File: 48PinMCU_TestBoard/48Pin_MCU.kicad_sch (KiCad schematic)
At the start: 33 parts, among them IC1 74LVC1G157GW,125, J4 SWD, J5 SWD, SW1 Reset, SW2 SW_SPDT, U1 STM32G431CBT6, Y1 Crystal

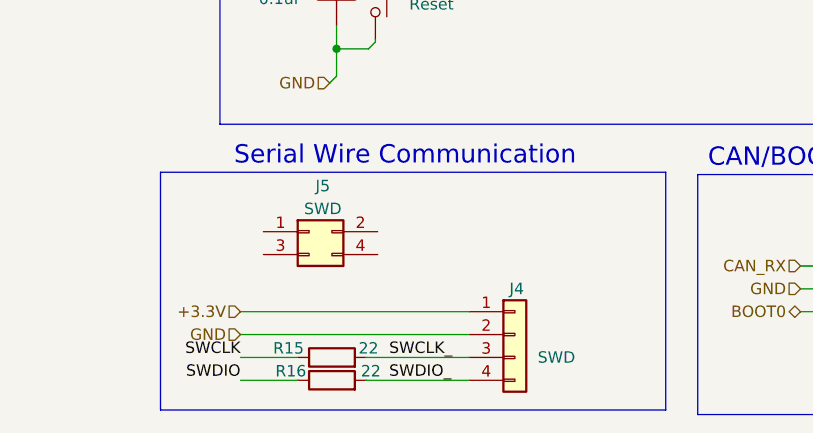
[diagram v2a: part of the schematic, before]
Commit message: made more changes!!
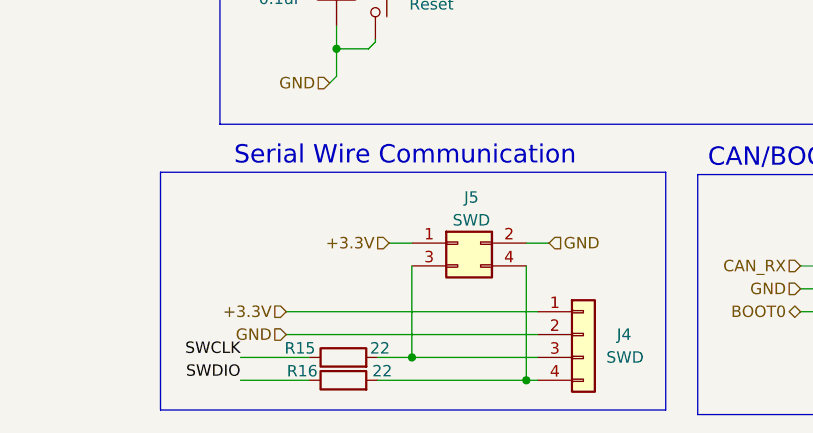
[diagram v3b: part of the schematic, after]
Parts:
- J5: footprint (none) -> UTSVT_Connectors:CONN04_878320406_MOL
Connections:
- net SWCLK_ is gone; now on an unnamed net: J4.3 (Pin_3), R15.2
- net SWDIO_ is gone; now on an unnamed net: J4.4 (Pin_4), R16.2
- net +3.3V: now also J5.1 (Pin_1)
- net GND: now also J5.2 (Pin_2)
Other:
- moved on the sheet: J4, J5, R15, R16
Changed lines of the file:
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@@
 	)
 	(junction
+		(at 186.69 157.48)
+		(diameter 0)
+		(color 0 0 0 0)
+	)
+	(junction
 		(at 220.726 46.736)
 		(diameter 0)
@@
 	)
 	(junction
+		(at 199.39 160.02)
+		(diameter 0)
+		(color 0 0 0 0)
+	)
+	(junction
 		(at 178.308 110.49)
 		(diameter 0)
@@
 	(wire
 		(pts
+			(xy 184.15 144.78) (xy 186.69 144.78)
+		)
+		(stroke
+			(width 0)
+			(type default)
+		)
+	)
+	(wire
+		(pts
 			(xy 171.704 45.212) (xy 173.228 46.736)
 		)
@@
 	(wire
 		(pts
-			(xy 173.99 160.02) (xy 167.64 160.02)
+			(xy 175.26 160.02) (xy 167.64 160.02)
 		)
 		(stroke
@@
 	(wire
 		(pts
-			(xy 167.64 154.94) (xy 193.04 154.94)
+			(xy 172.72 154.94) (xy 200.66 154.94)
 		)
 		(stroke
@@
 	(wire
 		(pts
+			(xy 199.39 147.32) (xy 199.39 160.02)
+		)
+		(stroke
+			(width 0)
+			(type default)
+		)
+	)
+	(wire
+		(pts
 			(xy 83.312 125.73) (xy 81.28 123.698)
 		)
@@
 	(wire
 		(pts
-			(xy 181.61 160.02) (xy 193.04 160.02)
+			(xy 182.88 160.02) (xy 199.39 160.02)
 		)
 		(stroke
@@
 	(wire
 		(pts
+			(xy 199.39 160.02) (xy 200.66 160.02)
+		)
+		(stroke
+			(width 0)
+			(type default)
+		)
+	)
+	(wire
+		(pts
 			(xy 248.92 107.95) (xy 250.19 109.22)
 		)
@@
 	(wire
 		(pts
+			(xy 186.69 147.32) (xy 186.69 157.48)
+		)
+		(stroke
+			(width 0)
+			(type default)
+		)
+	)
+	(wire
+		(pts
 			(xy 182.626 111.506) (xy 181.61 110.49)
 		)
@@
 	(wire
 		(pts
+			(xy 186.69 157.48) (xy 200.66 157.48)
+		)
+		(stroke
+			(width 0)
+			(type default)
+		)
+	)
+	(wire
+		(pts
 			(xy 172.72 71.12) (xy 186.69 71.12)
 		)
@@
 	(wire
 		(pts
-			(xy 173.99 157.48) (xy 167.64 157.48)
+			(xy 175.26 157.48) (xy 167.64 157.48)
 		)
 		(stroke
@@
 	(wire
 		(pts
-			(xy 181.61 157.48) (xy 193.04 157.48)
+			(xy 182.88 157.48) (xy 186.69 157.48)
 		)
 		(stroke
@@
 	(wire
 		(pts
-			(xy 167.64 152.4) (xy 193.04 152.4)
+			(xy 172.72 152.4) (xy 200.66 152.4)
 		)
 		(stroke
@@
 	(wire
 		(pts
+			(xy 199.39 144.78) (xy 201.93 144.78)
+		)
+		(stroke
+			(width 0)
+			(type default)
+		)
+	)
+	(wire
+		(pts
 			(xy 137.414 96.52) (xy 141.986 96.52)
 		)
@@
 		)
 	)
-	(label "SWDIO_"
-		(at 184.15 160.02 0)
-		(effects
-			(font
-				(size 1.27 1.27)
-			)
-			(justify left bottom)
-		)
-	)
 	(label "CAN_RX{slash}BOOT0"
 		(at 271.78 152.4 180)
@@
 		)
 	)
-	(label "SWCLK_"
-		(at 184.15 157.48 0)
-		(effects
-			(font
-				(size 1.27 1.27)
-			)
-			(justify left bottom)
-		)
-	)
 	(label "SWDIO"
 		(at 24.13 71.12 0)
@@
 		)
 	)
+	(hierarchical_label "+3.3V"
+		(shape input)
+		(at 184.15 144.78 180)
+		(effects
+			(font
+				(size 1.27 1.27)
+			)
+			(justify right)
+		)
+	)
 	(hierarchical_label "GND"
 		(shape input)
@@
 	(hierarchical_label "GND"
 		(shape input)
-		(at 167.64 154.94 180)
+		(at 172.72 154.94 180)
 		(effects
 			(font
@@
 		)
 	)
+	(hierarchical_label "GND"
+		(shape input)
+		(at 201.93 144.78 0)
+		(effects
+			(font
+				(size 1.27 1.27)
+			)
+			(justify left)
+		)
+	)
 	(hierarchical_label "PA15"
 		(shape bidirectional)
@@
 	(hierarchical_label "+3.3V"
 		(shape input)
-		(at 167.64 152.4 180)
+		(at 172.72 152.4 180)
 		(effects
 			(font
@@
 	(symbol
 		(lib_id "Connector_Generic:Conn_02x02_Odd_Even")
-		(at 175.26 143.51 0)
+		(at 191.77 144.78 0)
 		(unit 1)
 		(exclude_from_sim no)
@@
 		(dnp no)
 		(property "Reference" "J5"
-			(at 176.784 138.43 0)
+			(at 193.294 139.7 0)
 			(effects
 				(font
@@
 		)
 		(property "Value" "SWD"
-			(at 176.784 140.97 0)
+			(at 193.294 142.24 0)
 			(effects
 				(font
@@
 			)
 		)
-		(property "Footprint" ""
-			(at 175.26 143.51 0)
+		(property "Footprint" "UTSVT_Connectors:CONN04_878320406_MOL"
+			(at 191.77 144.78 0)
 			(effects
 				(font
@@
 		)
 		(property "Datasheet" "~"
-			(at 175.26 143.51 0)
+			(at 191.77 144.78 0)
 			(effects
 				(font
@@
 		)
 		(property "Description" "Generic connector, double row, 02x02, odd/even pin numbering scheme (row 1 odd numbers, row 2 even numbers), script generated (kicad-library-utils/schlib/autogen/connector/)"
-			(at 175.26 143.51 0)
+			(at 191.77 144.78 0)
 			(effects
 				(font
@@
 	(symbol
 		(lib_id "Connector_Generic:Conn_01x04")
-		(at 198.12 154.94 0)
+		(at 205.74 154.94 0)
 		(unit 1)
 		(exclude_from_sim no)
@@
 		(dnp no)
 		(property "Reference" "J4"
-			(at 199.136 149.86 0)
+			(at 211.074 154.94 0)
 			(effects
 				(font
@@
 		)
 		(property "Value" "SWD"
-			(at 200.66 157.4799 0)
+			(at 208.28 157.4799 0)
 			(effects
 				(font
@@
 		)
 		(property "Footprint" "Connector_PinHeader_2.54mm:PinHeader_1x04_P2.54mm_Vertical"
-			(at 198.12 154.94 0)
+			(at 205.74 154.94 0)
 			(effects
 				(font
@@
 		)
 		(property "Datasheet" "~"
-			(at 198.12 154.94 0)
+			(at 205.74 154.94 0)
 			(effects
 				(font
@@
 		)
 		(property "Description" "Generic connector, single row, 01x04, script generated (kicad-library-utils/schlib/autogen/connector/)"
-			(at 198.12 154.94 0)
+			(at 205.74 154.94 0)
 			(effects
 				(font
@@
 	(symbol
 		(lib_id "Device:R")
-		(at 177.8 157.48 90)
+		(at 179.07 157.48 90)
 		(unit 1)
 		(exclude_from_sim no)
@@
 		(dnp no)
 		(property "Reference" "R15"
-			(at 172.974 156.464 90)
+			(at 174.244 156.464 90)
 			(effects
 				(font
@@
 		)
 		(property "Value" "22"
-			(at 181.864 156.464 90)
+			(at 183.134 156.464 90)
 			(effects
 				(font
@@
 		)
 		(property "Footprint" "Resistor_SMD:R_0603_1608Metric_Pad0.98x0.95mm_HandSolder"
-			(at 177.8 159.258 90)
+			(at 179.07 159.258 90)
 			(effects
 				(font
@@
 		)
 		(property "Datasheet" "~"
-			(at 177.8 157.48 0)
+			(at 179.07 157.48 0)
 			(effects
 				(font
@@
 		)
 		(property "Description" "Resistor"
-			(at 177.8 157.48 0)
+			(at 179.07 157.48 0)
 			(effects
 				(font
@@
 		)
 		(property "LCSC P/N" "C25804"
-			(at 177.8 157.48 90)
+			(at 179.07 157.48 90)
 			(effects
 				(font
@@
 		)
 		(property "P/N" "FRC0603F22R0TS"
-			(at 177.8 157.48 90)
+			(at 179.07 157.48 90)
 			(effects
 				(font
@@
 	(symbol
 		(lib_id "Device:R")
-		(at 177.8 160.02 90)
+		(at 179.07 160.02 90)
 		(unit 1)
 		(exclude_from_sim no)
@@
 		(dnp no)
 		(property "Reference" "R16"
-			(at 173.228 159.004 90)
+			(at 174.498 159.004 90)
 			(effects
 				(font
@@
 		)
 		(property "Value" "22"
-			(at 182.118 159.004 90)
+			(at 183.388 159.004 90)
 			(effects
 				(font
@@
 		)
 		(property "Footprint" "Resistor_SMD:R_0603_1608Metric_Pad0.98x0.95mm_HandSolder"
-			(at 177.8 161.798 90)
+			(at 179.07 161.798 90)
 			(effects
 				(font
@@
 		)
 		(property "Datasheet" "~"
-			(at 177.8 160.02 0)
+			(at 179.07 160.02 0)
 			(effects
 				(font
@@
 		)
 		(property "Description" "Resistor"
-			(at 177.8 160.02 0)
+			(at 179.07 160.02 0)
 			(effects
 				(font
@@
 		)
 		(property "LCSC P/N" "C25804"
-			(at 177.8 160.02 90)
+			(at 179.07 160.02 90)
 			(effects
 				(font
@@
 		)
 		(property "P/N" "FRC0603F22R0TS"
-			(at 177.8 160.02 90)
+			(at 179.07 160.02 90)
 			(effects
 				(font
